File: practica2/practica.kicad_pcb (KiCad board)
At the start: 2 copper layers, 35.6 x 31.8 mm, 11 parts, among them Q1 BC549, Q2 BC549

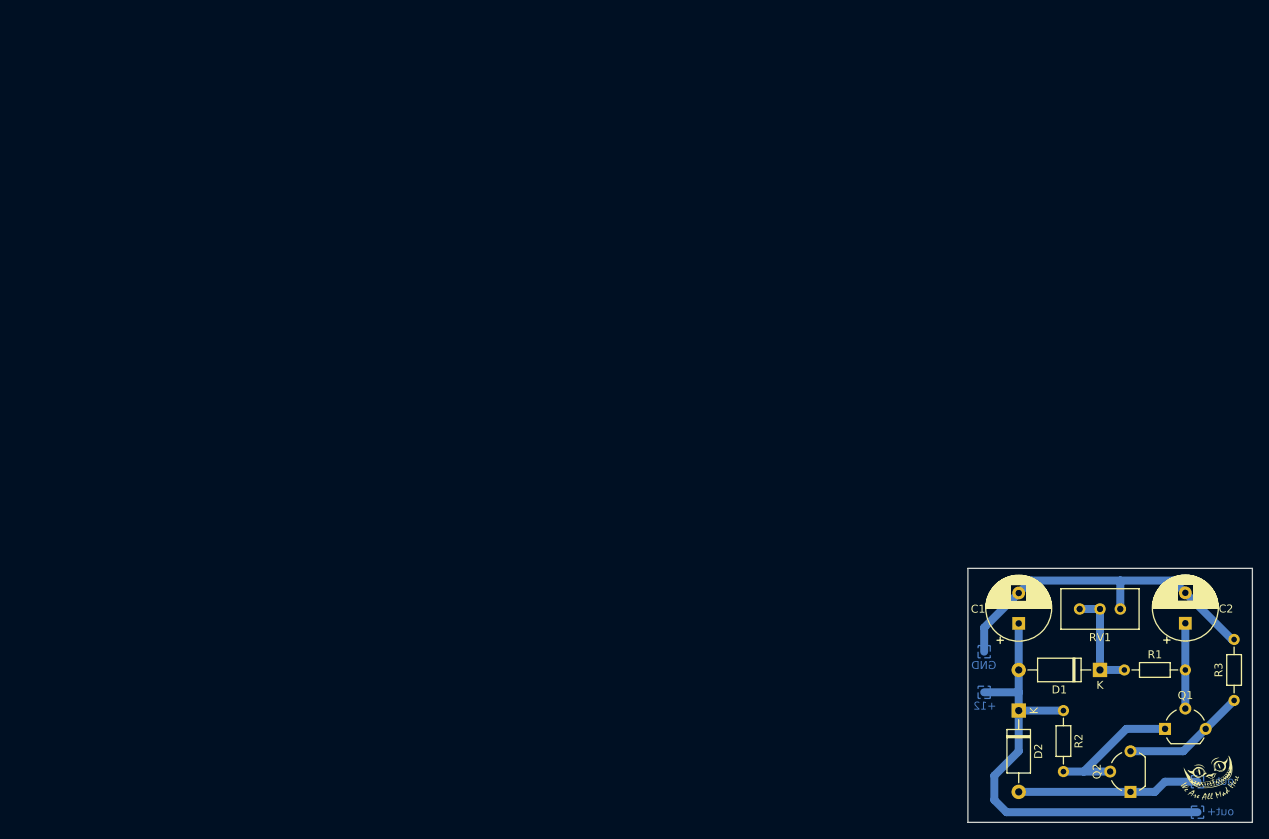
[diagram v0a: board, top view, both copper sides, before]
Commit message: 1
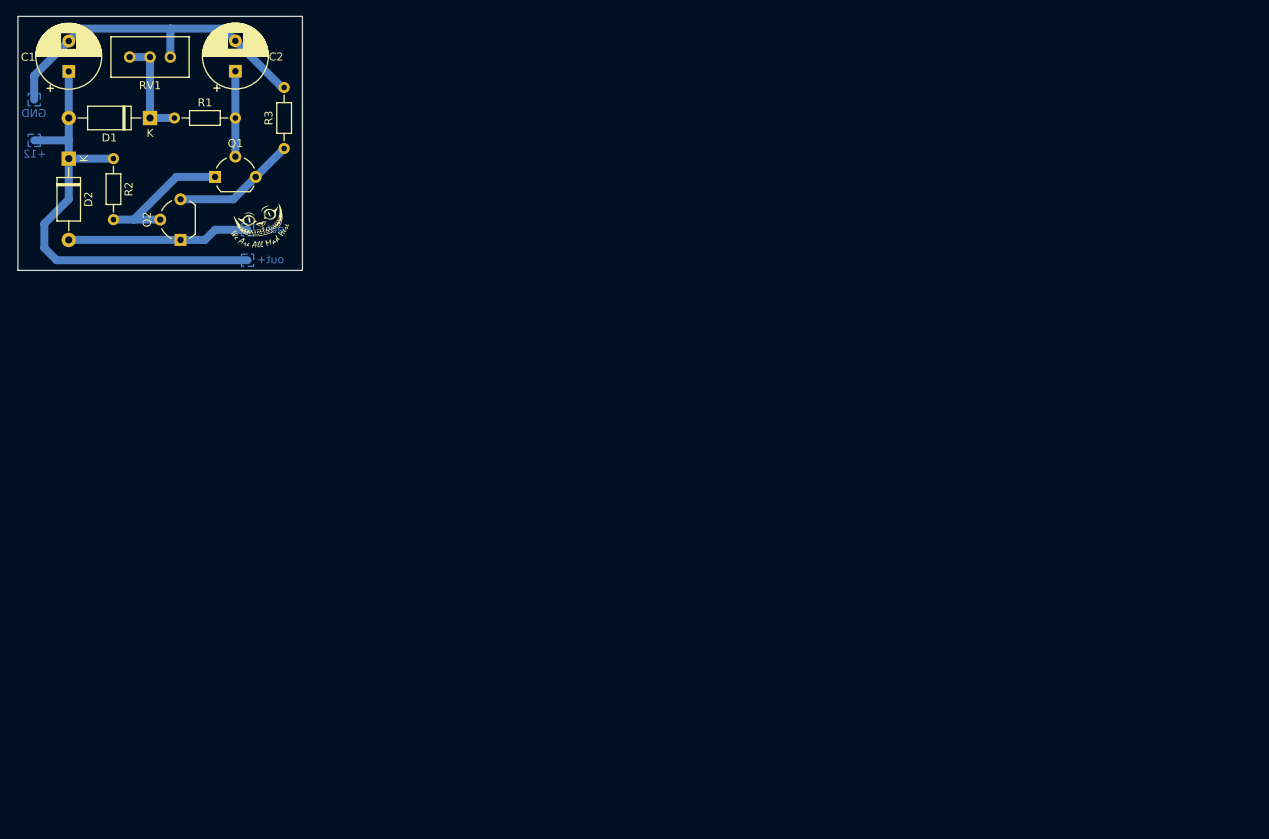
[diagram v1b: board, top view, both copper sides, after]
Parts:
- moved C1 137.3 mm to (18.4, 19.2)
- moved C2 137.3 mm to (39.2, 19.1)
- moved D2 137.3 mm to (18.4, 30.1)
- moved G*** 137.3 mm to (42.3, 38.7)
- moved Q1 137.3 mm to (36.7, 32.4)
- moved Q2 137.3 mm to (32.4, 40.2)
- moved R3 137.3 mm to (45.3, 28.8)
- moved RV1 137.3 mm to (26.0, 17.4)
- moved D1 137.3 mm to (28.6, 25.0)
- moved R1 137.3 mm to (31.6, 25.0)
- moved R2 137.3 mm to (24.0, 30.1)

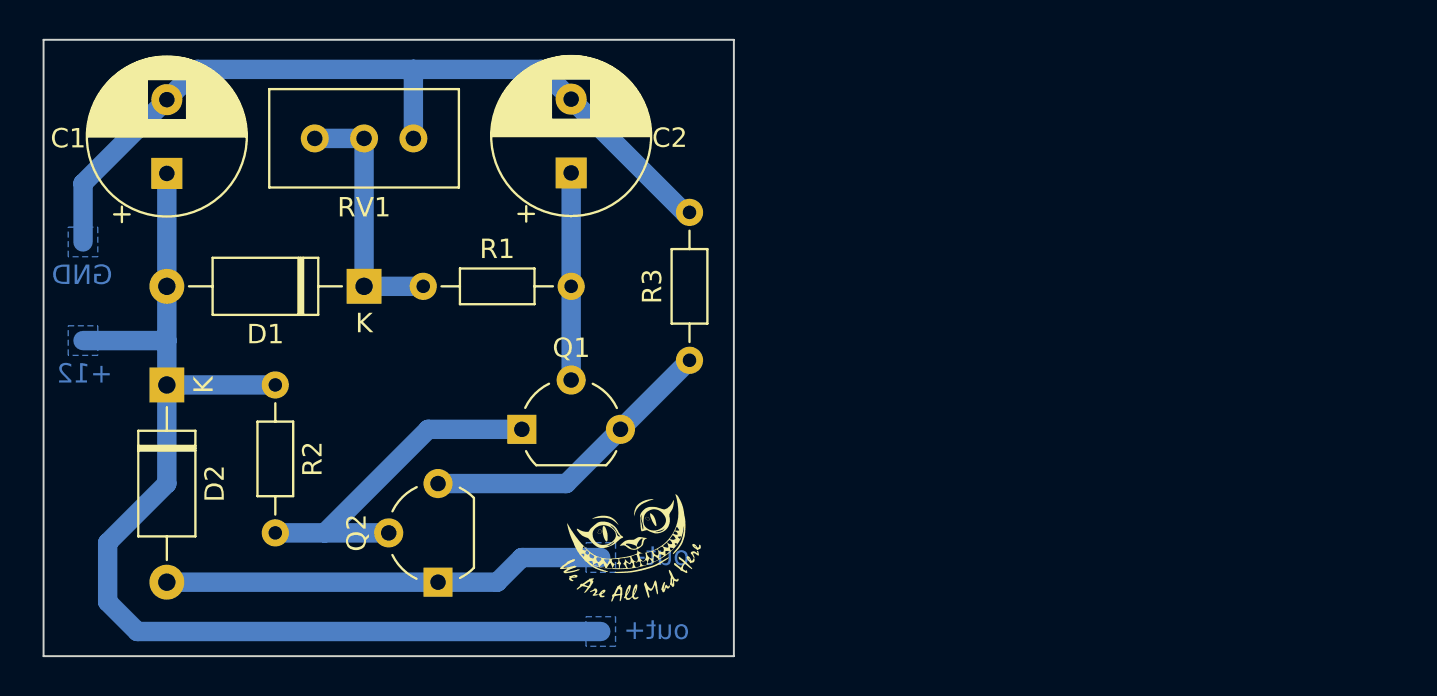
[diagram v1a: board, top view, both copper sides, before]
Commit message: 1
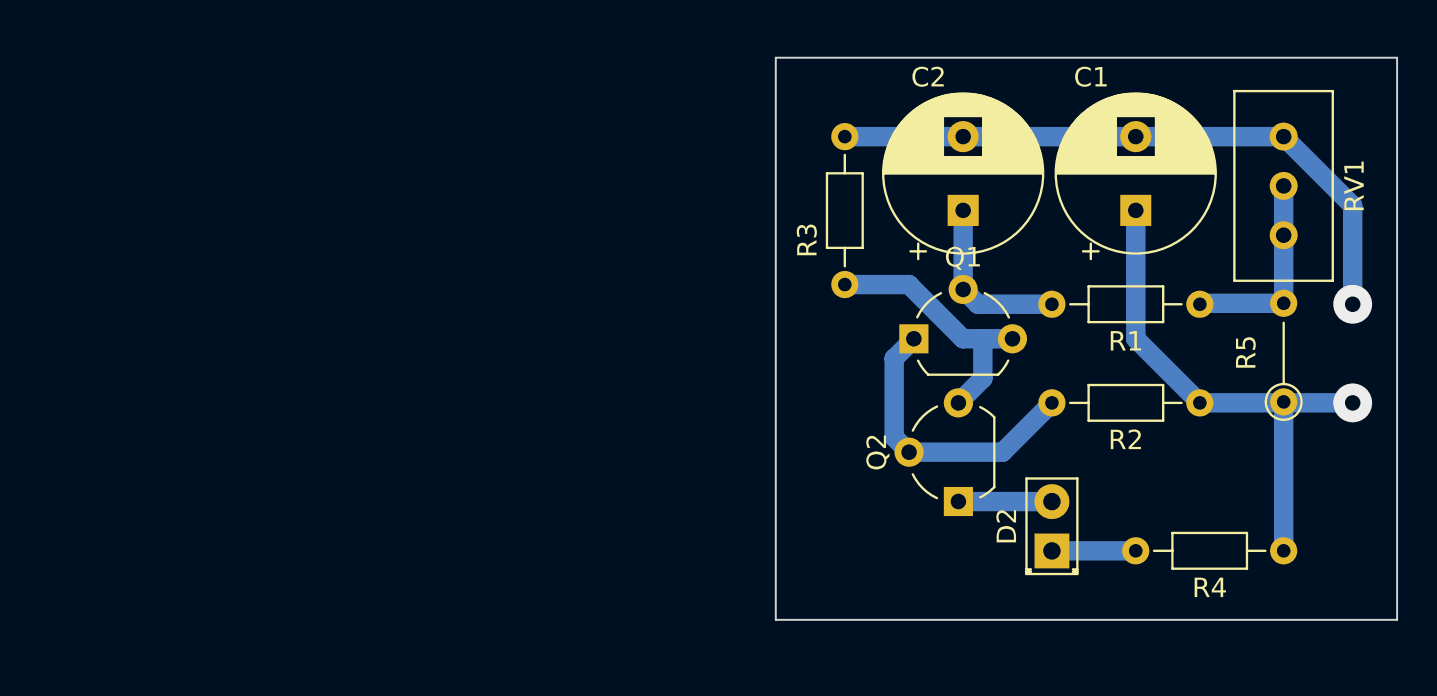
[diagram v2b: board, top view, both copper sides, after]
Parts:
- removed D1: GL5516, Diode_THT:D_A-405_P10.16mm_Horizontal
- removed G***: LOGO, LOGO
- added R4: 33, Resistor_THT:R_Axial_DIN0204_L3.6mm_D1.6mm_P7.62mm_Horizontal, F.Cu at (75.9, 38.6)
- added R5: R_Photo, Resistor_THT:R_Axial_DIN0204_L3.6mm_D1.6mm_P5.08mm_Vertical, F.Cu at (75.9, 30.9)
- D2: value 1N4148 -> LED; footprint Diode_THT:D_A-405_P10.16mm_Horizontal -> LED_THT:LED_D2.0mm_W4.8mm_H2.5mm_FlatTop
- moved RV1 50.2 mm to (75.9, 22.4), turned to -90 degrees
- moved C1 49.9 mm to (68.3, 21.1)
- moved R2 47.6 mm to (71.6, 31.0), turned to 180 degrees
- moved D2 46.4 mm to (64.0, 38.6), turned to 90 degrees
- moved R1 40.0 mm to (71.6, 25.9), turned to 180 degrees
- moved Q2 27.1 mm to (59.2, 36.1)
- moved Q1 20.7 mm to (56.9, 27.7)
- moved C2 20.3 mm to (59.4, 21.1)
- moved R3 8.90 mm to (53.3, 24.9)
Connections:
- net /out- renamed Net-(D2-A)
- D2 pad 1: +12V -> Net-(D2-K)
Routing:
- net +12V: track 59.3 -> 26.9 mm, vias 0 -> 1
- net Net-(D2-A): track 22.9 -> 4.82 mm
- net GND: track 43.3 -> 32.7 mm, vias 0 -> 1
- net Net-(D2-K): track 0.00 -> 4.32 mm
- net Net-(Q1-C): track 18.2 -> 15.0 mm
- net Net-(R1-Pad1): track 13.2 -> 10.4 mm
- net Net-(Q1-E): track 15.6 -> 13.6 mm
- net Net-(Q1-B): track 10.7 -> 8.96 mm
- removed copper zone on B.Cu, net +12V
- removed copper zone on B.Cu, net GND
- removed copper zone on B.Cu, net Net-(D2-A)
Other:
- board size 35.6 x 31.8 mm -> 32 x 29 mm
- board text removed: "+12"
- board text removed: "GND"
- board text removed: "out+"
- board text removed: "out-"

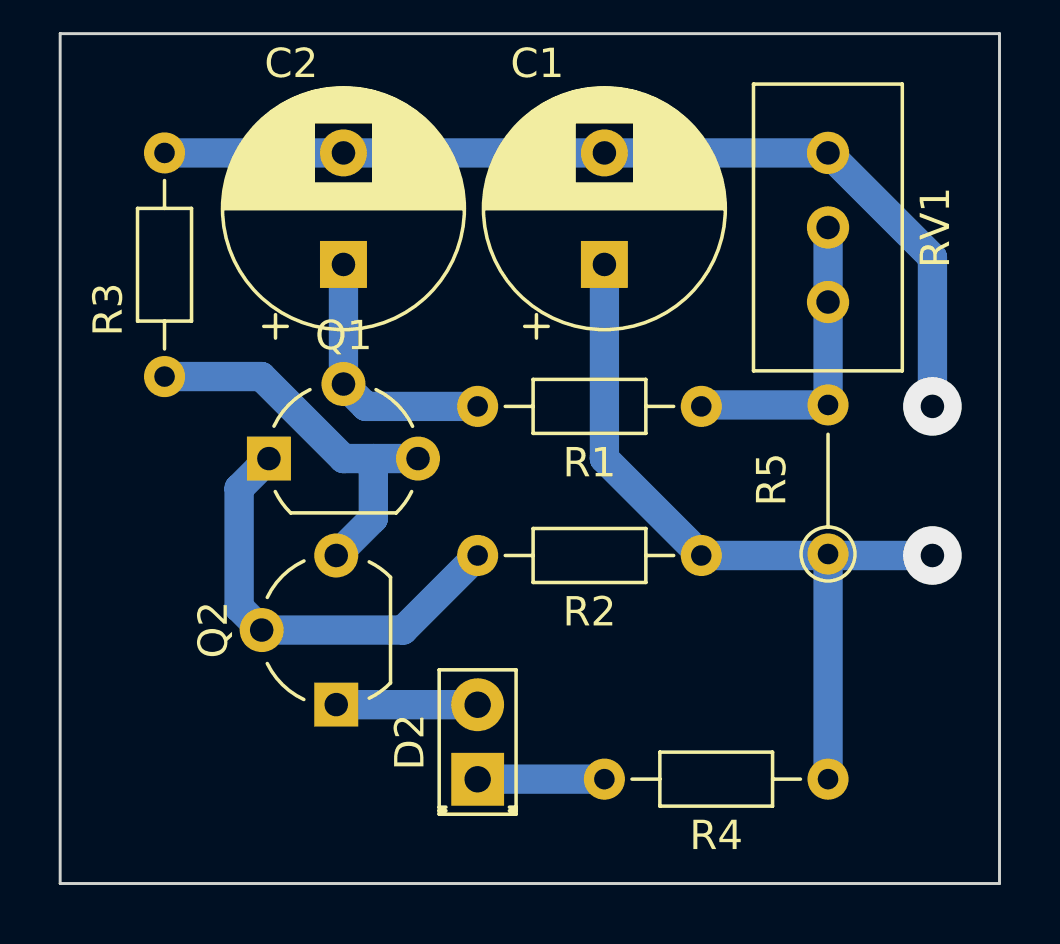
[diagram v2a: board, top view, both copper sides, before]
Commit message: 1
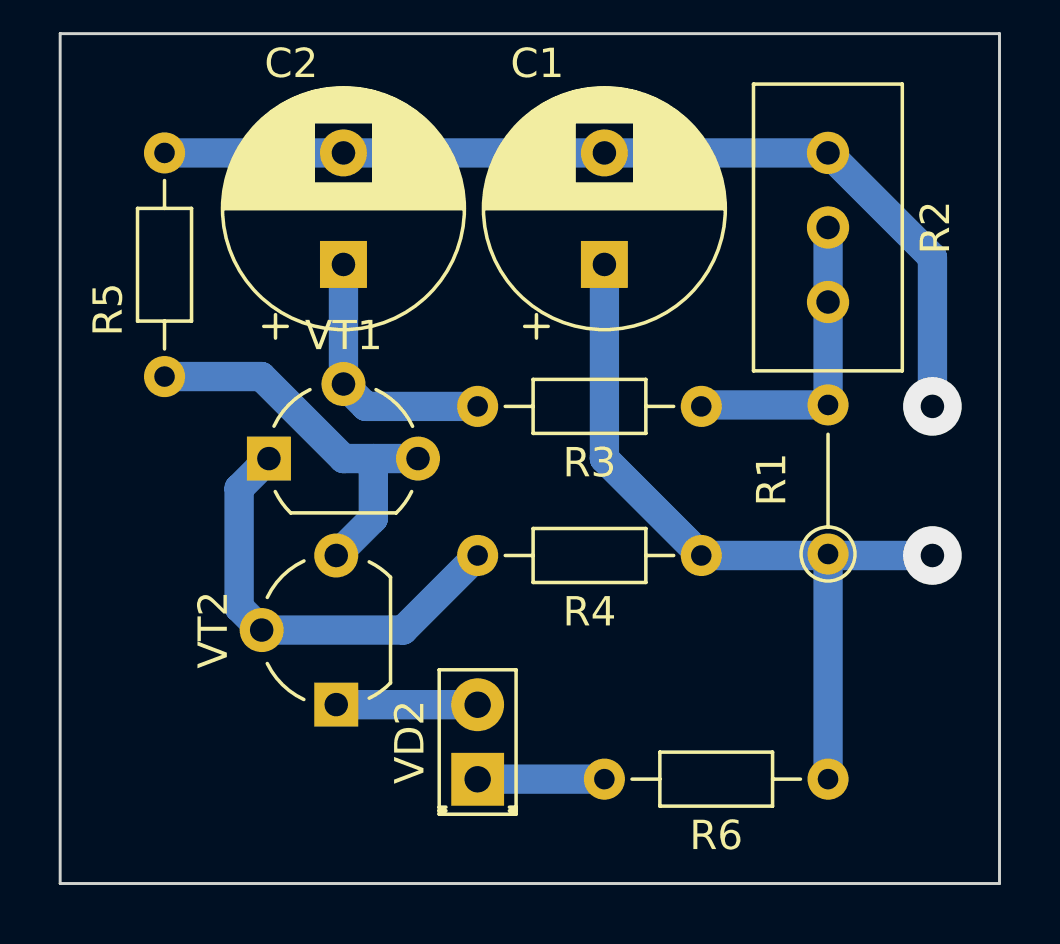
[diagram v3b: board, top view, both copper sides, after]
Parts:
- R1: renamed from R5; value R_Photo -> GL5516
- renumbered RV1 to R2, R1 to R3, R2 to R4, R3 to R5, R4 to R6, D2 to VD2, Q1 to VT1, Q2 to VT2
